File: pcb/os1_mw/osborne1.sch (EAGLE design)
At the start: 2 parts

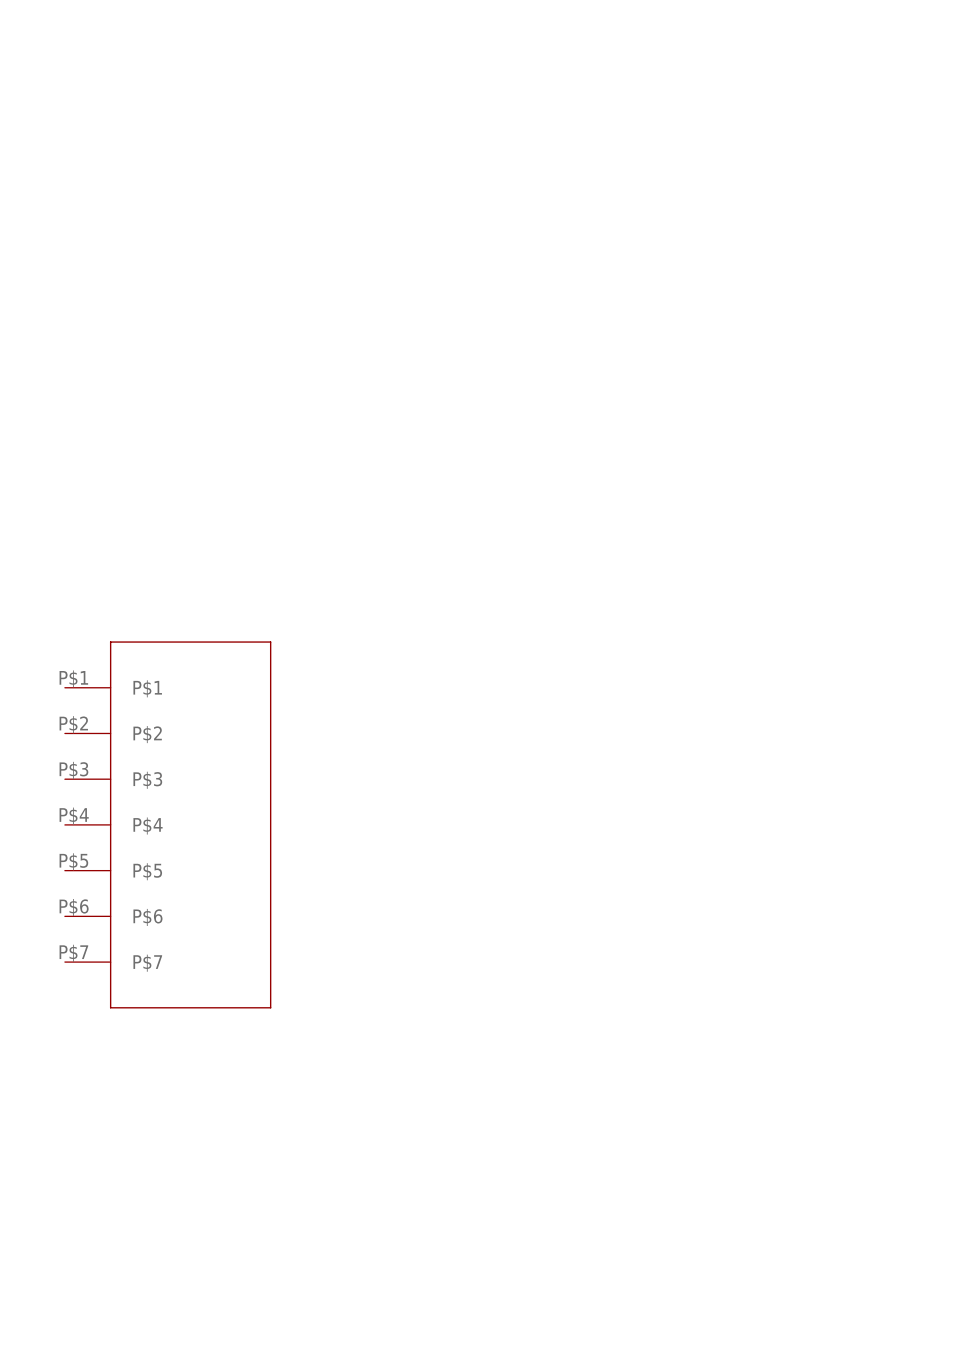
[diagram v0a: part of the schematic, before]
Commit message: added docs
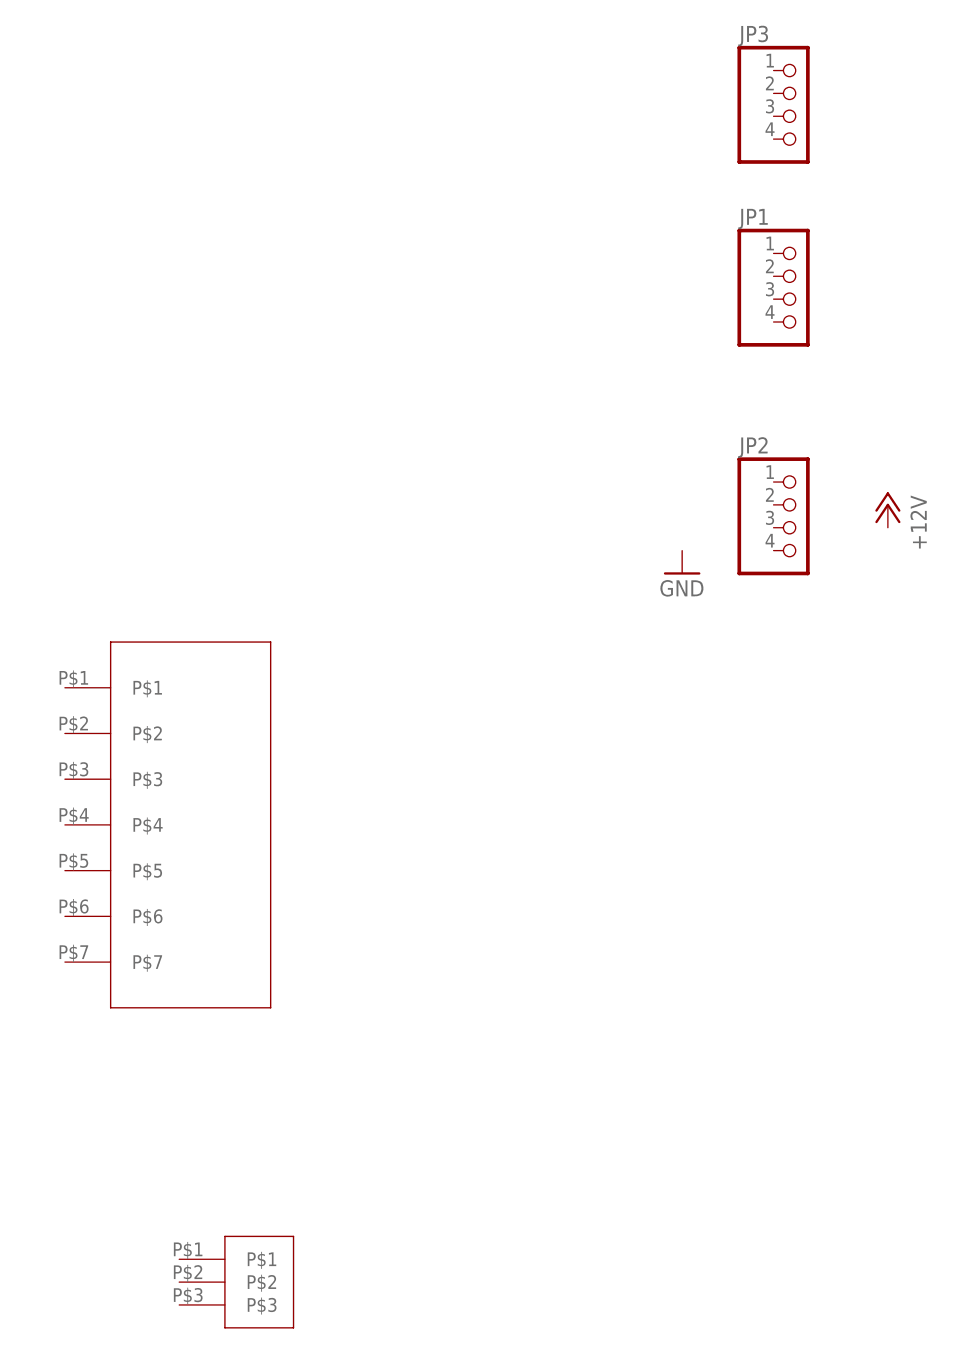
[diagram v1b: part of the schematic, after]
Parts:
- added JP1, JP2, JP3: (no value), pinhead:PINHD-1X4/90
- added U$3: VH396_3P, 396_conn:VH396_3P
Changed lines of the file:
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@@
 <part name="U$1" library="apricot" deviceset="MEANWELL_RD50" device=""/>
 <part name="U$2" library="os1" deviceset="TERM9.5" device=""/>
+<part name="U$3" library="396_conn" deviceset="VH396_3P" device=""/>
+<part name="JP2" library="pinhead" library_urn="urn:adsk.eagle:library:325" deviceset="PINHD-1X4" device="/90" package3d_urn="urn:adsk.eagle:package:22404/2"/>
+<part name="P+4" library="supply1" library_urn="urn:adsk.eagle:library:371" deviceset="+12V" device=""/>
+<part name="GND17" library="supply1" library_urn="urn:adsk.eagle:library:371" deviceset="GND" device=""/>
+<part name="JP1" library="pinhead" library_urn="urn:adsk.eagle:library:325" deviceset="PINHD-1X4" device="/90" package3d_urn="urn:adsk.eagle:package:22404/2"/>
+<part name="JP3" library="pinhead" library_urn="urn:adsk.eagle:library:325" deviceset="PINHD-1X4" device="/90" package3d_urn="urn:adsk.eagle:package:22404/2"/>
 </parts>
 <sheets>
@@
 <instance part="U$1" gate="G$1" x="45.72" y="38.1" smashed="yes"/>
 <instance part="U$2" gate="G$1" x="109.22" y="43.18" smashed="yes"/>
+<instance part="U$3" gate="G$1" x="111.76" y="-7.62" smashed="yes"/>
+<instance part="JP2" gate="A" x="175.26" y="73.66" smashed="yes">
+<attribute name="NAME" x="168.91" y="81.915" size="1.778" layer="95"/>
+<attribute name="VALUE" x="168.91" y="66.04" size="1.778" layer="96"/>
+</instance>
+<instance part="P+4" gate="1" x="185.42" y="76.2" smashed="yes" rot="MR0">
+<attribute name="VALUE" x="187.96" y="71.12" size="1.778" layer="96" rot="MR90"/>
+</instance>
+<instance part="GND17" gate="1" x="162.56" y="68.58" smashed="yes">
+<attribute name="VALUE" x="160.02" y="66.04" size="1.778" layer="96"/>
+</instance>
+<instance part="JP1" gate="A" x="175.26" y="99.06" smashed="yes">
+<attribute name="NAME" x="168.91" y="107.315" size="1.778" layer="95"/>
+<attribute name="VALUE" x="168.91" y="91.44" size="1.778" layer="96"/>
+</instance>
+<instance part="JP3" gate="A" x="175.26" y="119.38" smashed="yes">
+<attribute name="NAME" x="168.91" y="127.635" size="1.778" layer="95"/>
+<attribute name="VALUE" x="168.91" y="111.76" size="1.778" layer="96"/>
+</instance>
 </instances>
 <busses>
@@
 which will not be processed correctly with this version.
 </note>
+<note version="8.2" severity="warning">
+Since Version 8.2, EAGLE supports online libraries. The ids
+of those online libraries will not be understood (or retained)
+with this version.
+</note>
+<note version="8.3" severity="warning">
+Since Version 8.3, EAGLE supports URNs for individual library
+assets (packages, symbols, and devices). The URNs of those assets
+will not be understood (or retained) with this version.
+</note>
+<note version="8.3" severity="warning">
+Since Version 8.3, EAGLE supports the association of 3D packages
+with devices in libraries, schematics, and board files. Those 3D
+packages will not be understood (or retained) with this version.
+</note>
 </compatibility>

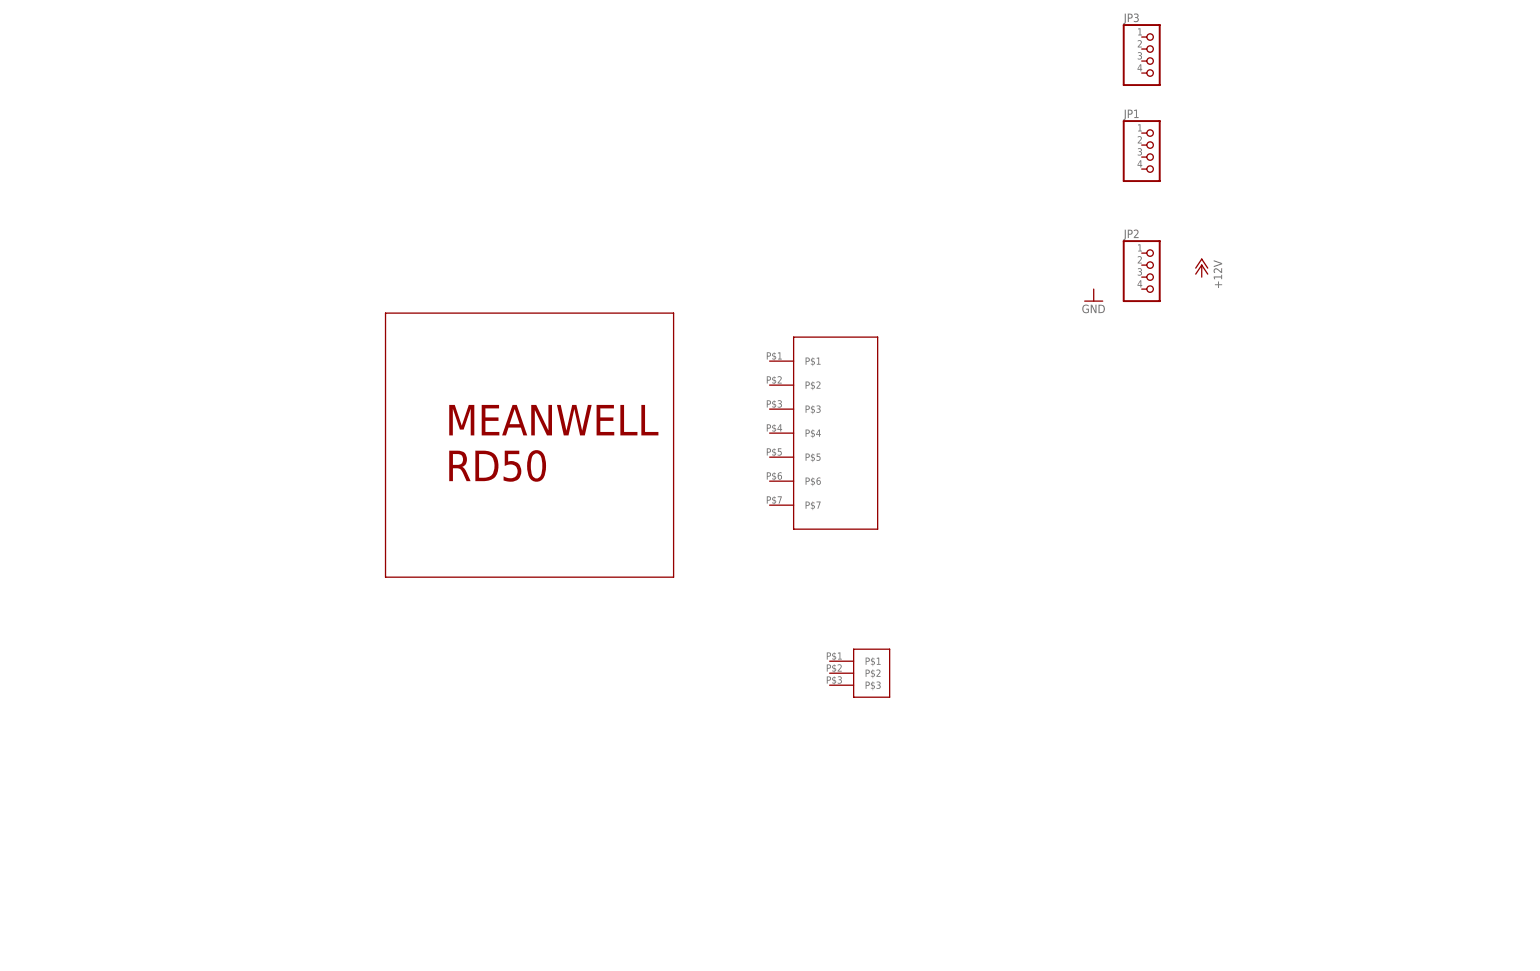
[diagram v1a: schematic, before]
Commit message: new os1 pcb done
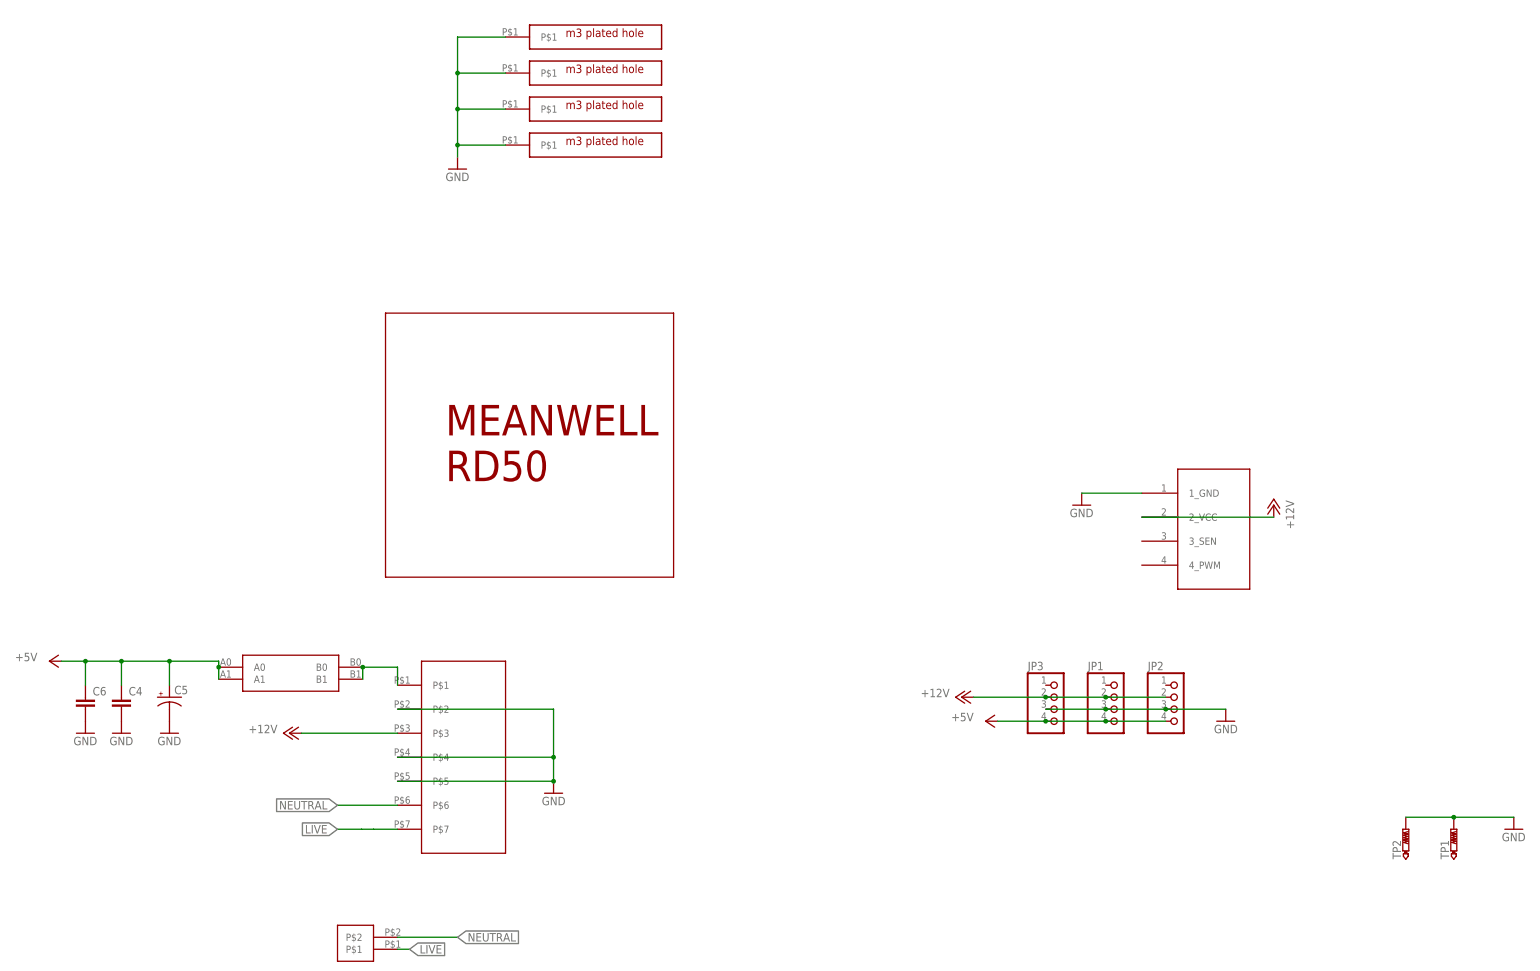
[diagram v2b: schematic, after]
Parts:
- removed U$3: VH396_3P, 396_conn:VH396_3P
- added C4, C6: (no value), capacitor-wima:C5/2.5
- added C5: (no value), adafruit_changed:CPOL-USE3.5-8
- added JP4: (no value), appleii:4PIN_FAN
- added TP1, TP2: PTR1PAD1-17, testpad:PTR1PAD1-17
- added U$4, U$5, U$6, U$8: M3_HOLE_PLATED, os1:M3_HOLE_PLATED
- added U$7: 396_2P_LIVE, 396_conn:396_2P_LIVE
- added U$9: CAR_FUSE_HOLDER3IN1, atx_power_control:CAR_FUSE_HOLDER3IN1
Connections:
- new net +12V: JP1.2, JP2.2, JP3.2, JP4.2_VCC, U$2.P$3
- new net +5V: C4.1, C5.+, C6.1, JP1.4, JP2.4, JP3.4, U$9.A0, U$9.A1
- new net GND: C4.2, C5.-, C6.2, JP1.3, JP2.3, JP3.3, JP4.1_GND, TP1.TP, TP2.TP, U$2.P$2, U$2.P$4, U$2.P$5, U$4.P$1, U$5.P$1, U$6.P$1, U$8.P$1
- new net LIVE: U$2.P$7, U$7.P$1
- new net N$2: U$2.P$1, U$9.B0, U$9.B1
- new net NEUTRAL: U$2.P$6, U$7.P$2
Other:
- moved on the sheet: JP1, JP2, JP3
